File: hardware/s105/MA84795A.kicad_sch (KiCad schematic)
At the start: 9 parts, among them U4 case only

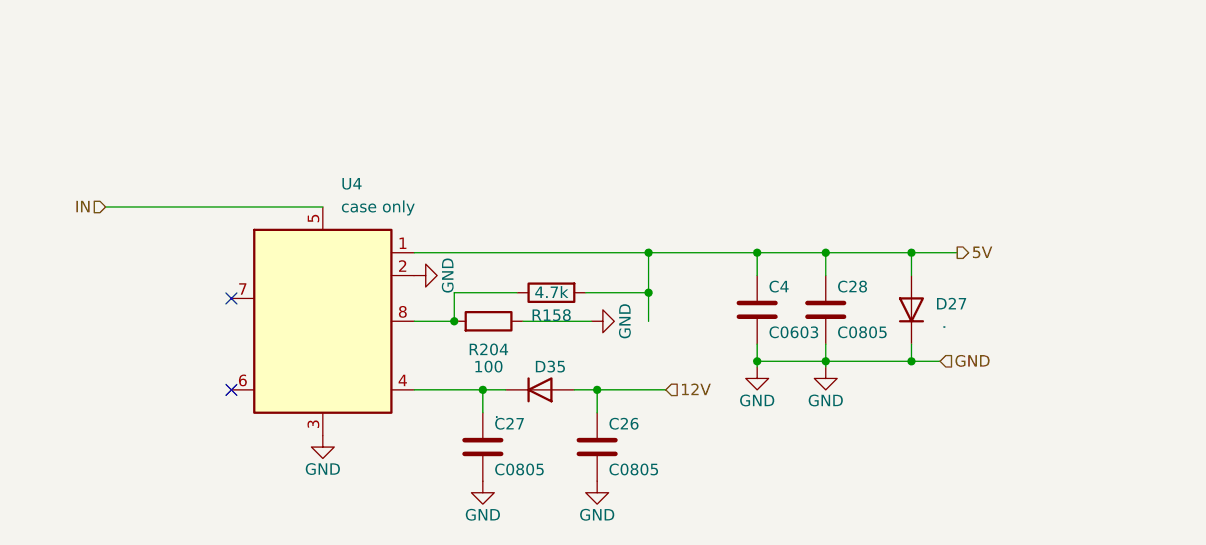
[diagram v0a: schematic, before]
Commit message: закончила пока что
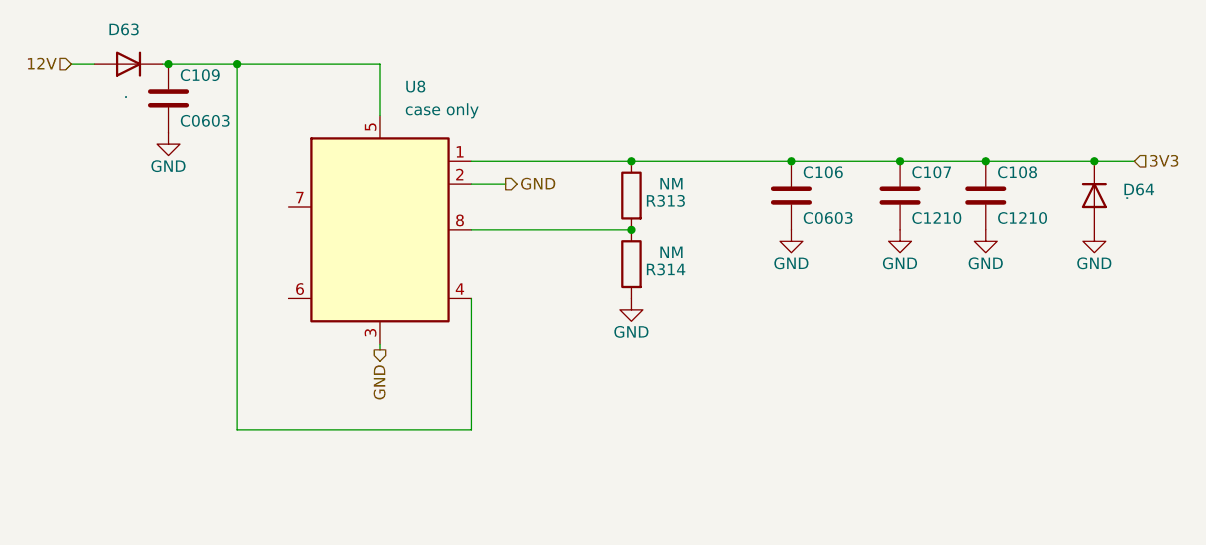
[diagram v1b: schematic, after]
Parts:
- removed C26, C27, C28: C0805, Capacitor_SMD:C_0805_2012Metric, symbol Device:C
- removed C4: C0603, Capacitor_SMD:C_0603_1608Metric, symbol Device:C
- removed D27: ., Diode_SMD:D_SMA, symbol Diode:US2JA
- removed D35: ., Diode_SMD:D_SOD-123, symbol Diode:1N4148W
- removed R158: 4.7k, Resistor_SMD:R_0603_1608Metric, symbol Device:R
- removed R204: 100, Resistor_SMD:R_0603_1608Metric, symbol Device:R
- removed U4: case only, Package_SO:SOIC-8_3.9x4.9mm_P1.27mm, symbol Regulator_Controller:L6727
- added C106, C109: C0603, Capacitor_SMD:C_0603_1608Metric, symbol Device:C
- added C107, C108: C1210, Capacitor_SMD:C_1210_3225Metric, symbol Device:C
- added D63, D64: ., Diode_SMD:D_SOD-123, symbol Diode:1N4148W
- added R313, R314: NM, Resistor_SMD:R_0603_1608Metric, symbol Device:R
- added U8: case only, Package_SO:SOIC-8_3.9x4.9mm_P1.27mm, symbol Regulator_Controller:L6727
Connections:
- net 12V: now also D63.2 (A)
- net GND: now also C106.2, C107.2, C108.2, C109.2, D64.2 (A), R314.2, U8.2 (UGATE), U8.3 (GND)
- new net: C109.1, D63.1 (K), U8.4 (LGATE), U8.5 (VCC)
- new net: R313.2, R314.1, U8.8 (PHASE)
- new net 3V3: C106.1, C107.1, C108.1, D64.1 (K), R313.1, U8.1 (BOOT)
- no-connect marks 2 -> 0

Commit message: #4 #5 #6 #8
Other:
- company: (none) -> rusEFI
- title: (none) -> s105
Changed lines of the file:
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@@
 (kicad_sch (version 20211123) (generator eeschema)
-  (paper "A4")
+  (paper "A3" portrait)
+  (title_block
+    (title "s105")
+    (rev "0.1")
+    (company "rusEFI")
+  )
   (junction (at 193.04 76.835) (diameter 0) (color 0 0 0 0)
   )
